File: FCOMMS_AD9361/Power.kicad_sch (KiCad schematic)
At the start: 16 parts, among them U201 LT8644SIV-TRMPBF

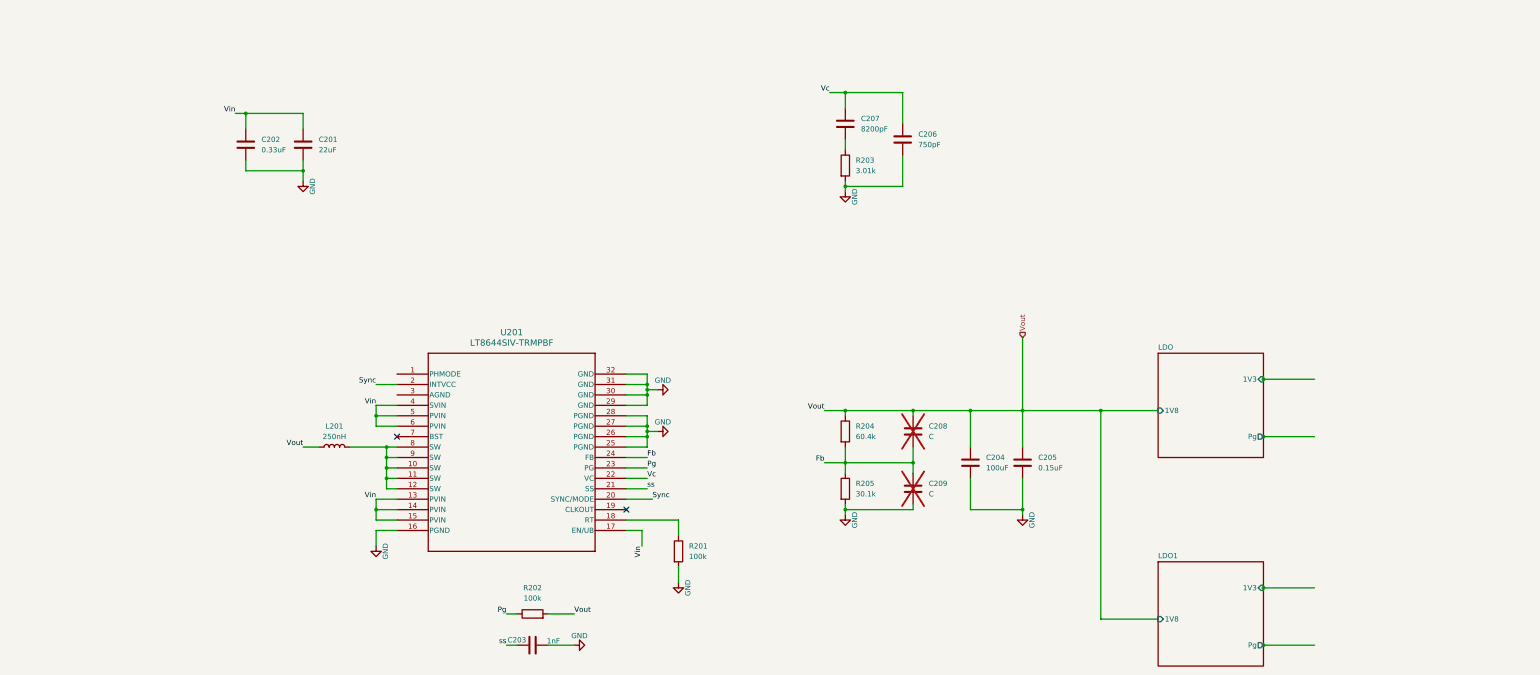
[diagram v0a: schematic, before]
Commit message: agile RF
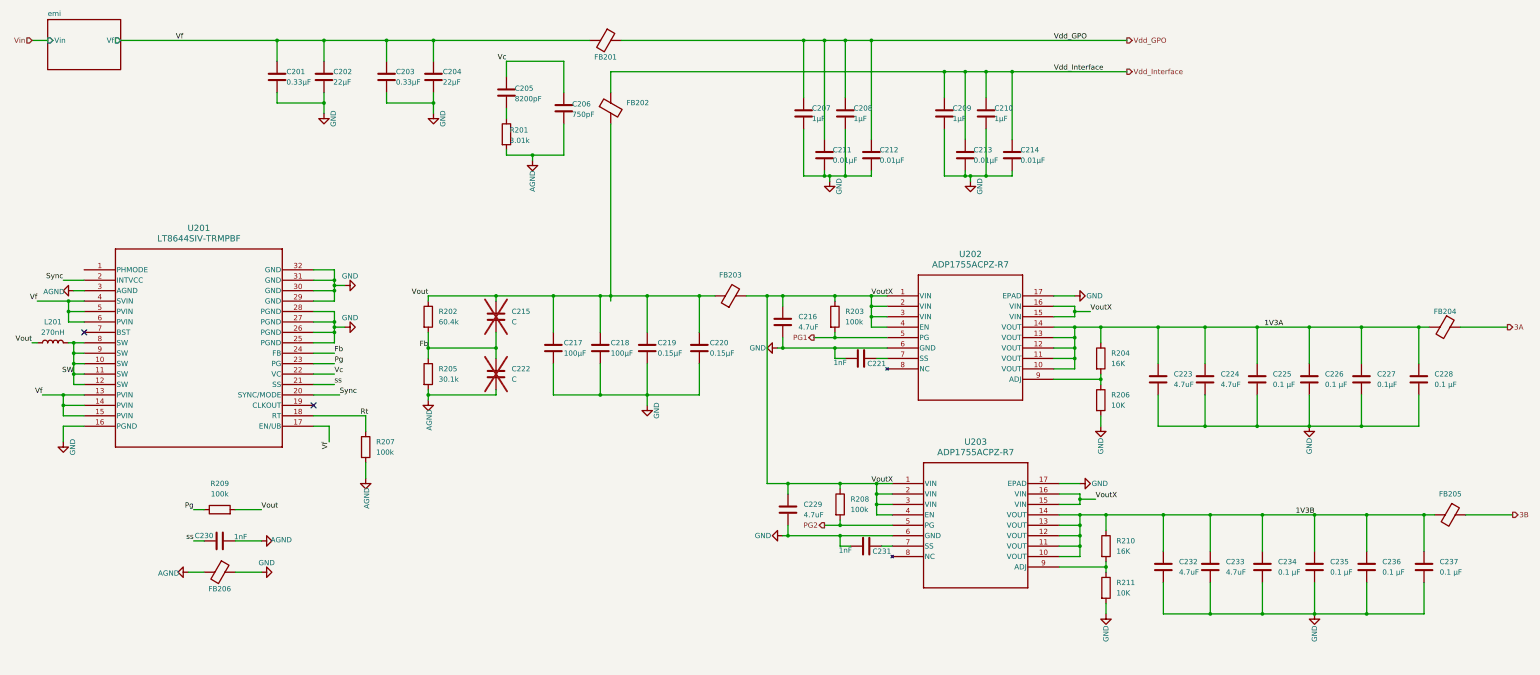
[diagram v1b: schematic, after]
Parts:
- added C203: 0.33µF, Capacitor_SMD:C_0603_1608Metric, symbol Device:C
- added C204: 22µF, Capacitor_SMD:C_0603_1608Metric, symbol Device:C
- added C207, C208, C209, C210: 1µF, Capacitor_SMD:C_0603_1608Metric, symbol Device:C
- added C211, C212, C213, C214: 0.01µF, Capacitor_SMD:C_0805_2012Metric, symbol Device:C
- added C216, C223, C224, C229, C232, C233: 4.7uF, Capacitor_SMD:C_0805_2012Metric, symbol Device:C
- added C217: 100µF, Capacitor_SMD:C_1206_3216Metric, symbol Device:C
- added C220: 0.15µF, Capacitor_SMD:C_0603_1608Metric, symbol Device:C
- added C221, C231: 1nF, Capacitor_SMD:C_0603_1608Metric, symbol Device:C
- added C225, C226, C228, C234, C235, C236, C237: 0.1 µF, Capacitor_SMD:C_0603_1608Metric, symbol Device:C
- added C227: 0.1µF, Capacitor_SMD:C_0603_1608Metric, symbol Device:C
- added FB201, FB206: 75 Ohms @ 100 MHz, Inductor_SMD:L_0603_1608Metric, symbol Device:FerriteBead
- added FB202, FB203, FB204, FB205: 30 Ohms @ 100 MHz, Inductor_SMD:L_0603_1608Metric, symbol Device:FerriteBead
- added R203, R208: 100k, Resistor_SMD:R_0603_1608Metric, symbol Device:R
- added R204, R210: 16K, Resistor_SMD:R_0603_1608Metric, symbol Device:R
- added R206, R211: 10K, Resistor_SMD:R_0603_1608Metric, symbol Device:R
- added U202, U203: ADP1755ACPZ-R7, Package_CSP:Analog_LFCSP-16-1EP_4x4mm_P0.65mm_EP2.1x2.1mm_ThermalVias, symbol ADP1755:ADP1755ACPZ-R7
- C201: renamed from C202; value 0.33uF -> 0.33µF
- C202: renamed from C201; value 22uF -> 22µF
- C218: renamed from C204; value 100uF -> 100µF
- C219: renamed from C205; value 0.15uF -> 0.15µF
- L201: value 250nH -> 270nH; footprint Inductor_SMD:L_12x12mm_H8mm -> Inductor_SMD:L_Coilcraft_XAL4040-XXX
- renumbered C207 to C205, C208 to C215, C209 to C222, C203 to C230, R203 to R201, R204 to R202, R201 to R207, R202 to R209
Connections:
- net GND: now also C203.2, C204.2, C207.2, C208.2, C209.2, C210.2, C211.2, C212.2, C213.2, C214.2, C216.2, C217.2, C220.2, C221.2, C223.2, C224.2, C225.2, C226.2, C227.2, C228.2, C229.2, C231.2, C232.2, C233.2, C234.2, C235.2, C236.2, C237.2, FB206.1, R206.2, R211.2, U202.17 (EPAD), U202.6 (GND), U203.17 (EPAD), U203.6 (GND); no longer C206.2, C222.2, C230.2, R201.2, R205.2, R207.2
- net Vin: no longer C201.1, C202.1, U201.13 (PVIN), U201.14 (PVIN), U201.15 (PVIN), U201.17 (EN/UB), U201.4 (SVIN), U201.5 (PVIN), U201.6 (PVIN)
- net Vout: now also C217.1, C220.1, FB202.2, FB203.1
- net Rt: now reaches R207.1, U201.18 (RT)
- net SW: now reaches L201.2, U201.10 (SW), U201.11 (SW), U201.12 (SW), U201.8 (SW), U201.9 (SW)
- net AGND: now reaches U201.3 (AGND)
- net AGND: now also C206.2, C222.2, C230.2, R201.2, R205.2, R207.2, FB206.2
- new net: R210.2, R211.1, U203.9 (ADJ)
- new net: C231.1, U203.7 (SS)
- new net: R204.2, R206.1, U202.9 (ADJ)
- new net: C221.1, U202.7 (SS)
- new net 1V3A: C223.1, C224.1, C225.1, C226.1, C227.1, C228.1, FB204.2, R204.1, U202.10 (VOUT), U202.11 (VOUT), U202.12 (VOUT), U202.13 (VOUT), U202.14 (VOUT)
- new net 1V3B: C232.1, C233.1, C234.1, C235.1, C236.1, C237.1, FB205.2, R210.1, U203.10 (VOUT), U203.11 (VOUT), U203.12 (VOUT), U203.13 (VOUT), U203.14 (VOUT)
- new net 3A: FB204.1
- new net 3B: FB205.1
- new net PG1: R203.2, U202.5 (PG)
- new net PG2: R208.2, U203.5 (PG)
- new net Vdd_GPO: C207.1, C208.1, C211.1, C212.1, FB201.1
- new net Vdd_Interface: C209.1, C210.1, C213.1, C214.1, FB202.1
- new net Vf: C201.1, C202.1, C203.1, C204.1, FB201.2, U201.13 (PVIN), U201.14 (PVIN), U201.15 (PVIN), U201.17 (EN/UB), U201.4 (SVIN), U201.5 (PVIN), U201.6 (PVIN)
- new net VoutX: C216.1, C229.1, FB203.2, R203.1, R208.1, U202.1 (VIN), U202.15 (VIN), U202.16 (VIN), U202.2 (VIN), U202.3 (VIN), U202.4 (EN), U203.1 (VIN), U203.15 (VIN), U203.16 (VIN), U203.2 (VIN), U203.3 (VIN), U203.4 (EN)
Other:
- removed sheet LDO
- removed sheet LDO1
- added sheet emi (emi.kicad_sch)
- moved on the sheet: C201, C202, C205, C206, C215, C218, C219, C222, C230, L201, R201, R202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

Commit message: add local library
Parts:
- C201, C202, C203, C204, C205, C206, C207, C208, C209, C210, C211, C212, C213, C214, C215, C216, C217, C218, C219, C220, C221, C222, C223, C224, C225, C226, C227, C228, C229, C230, C231, C232, C233, C234, C235, C236, C237: symbol Device:C -> Library:C
- FB201, FB202, FB203, FB204, FB205, FB206: symbol Device:FerriteBead -> Library:FerriteBead
- L201: symbol Device:L -> Library:L
- R201, R202, R203, R204, R205, R206, R207, R208, R209, R210, R211: symbol Device:R -> Library:R
- U201: symbol LT8644S:LT8644SIV-TRMPBF -> Library:LT8644SIV-TRMPBF
- U202, U203: symbol ADP1755:ADP1755ACPZ-R7 -> Library:ADP1755ACPZ-R7_1
